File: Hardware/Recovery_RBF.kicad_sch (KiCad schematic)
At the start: 8 parts, among them J6 RCV_SYS, J7 RBF_SYS, Q8 AO3400A

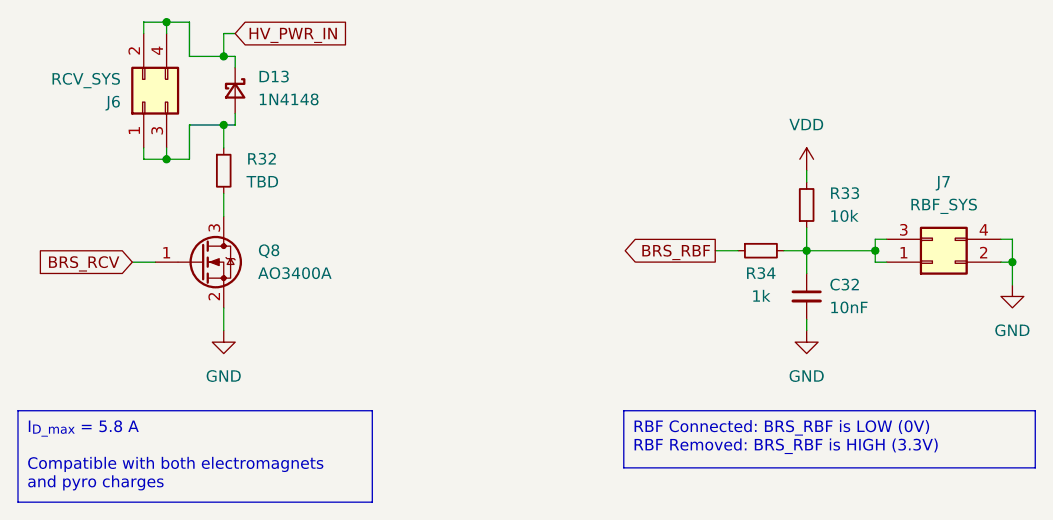
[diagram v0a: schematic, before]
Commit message: Developing HW - routing
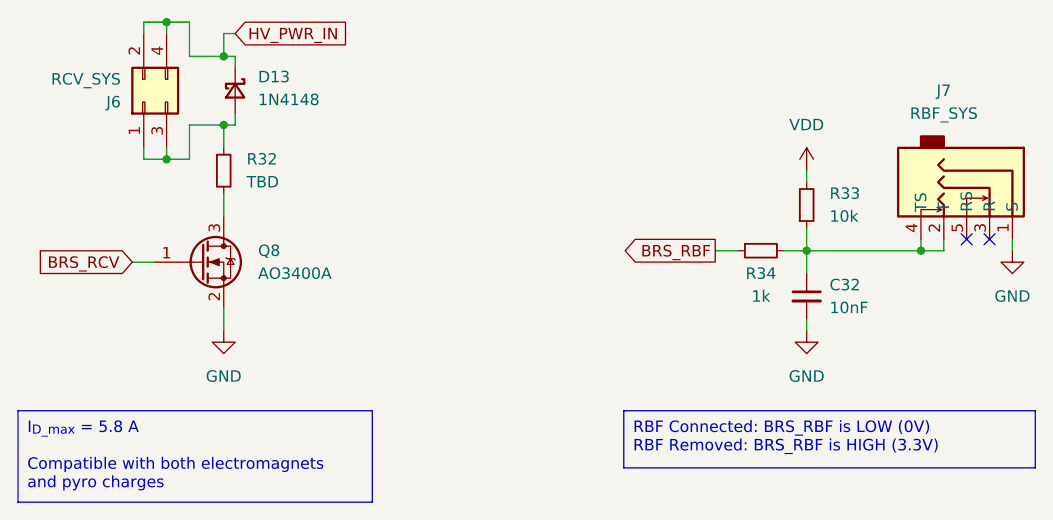
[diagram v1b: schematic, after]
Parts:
- J7: footprint Connector_Molex:Molex_Micro-Fit_3.0_43045-0412_2x02_P3.00mm_Vertical -> BRS_Footprints:AudioJack_Vertical; symbol Connector_Generic:Conn_02x02_Odd_Even -> BRS_Library:AudioJack_5pins
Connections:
- net GND: now also J7.1 (S); no longer J7.2 (Pin_2), J7.4 (Pin_4)
- net at C32.1, R33.1, R34.2: now also J7.2 (T), J7.4 (TS); no longer J7.1 (Pin_1), J7.3 (Pin_3)
- no-connect marks 0 -> 2
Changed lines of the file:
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@@
-	)
-	(junction
-		(at 191.77 101.6)
-		(diameter 0)
-		(color 0 0 0 0)
 	)
 	(junction
@@
 	)
 	(junction
-		(at 207.01 102.87)
-		(diameter 0)
-		(color 0 0 0 0)
-	)
-	(junction
 		(at 119.38 80.01)
 		(diameter 0)
 		(color 0 0 0 0)
 	)
+	(junction
+		(at 196.85 101.6)
+		(diameter 0)
+		(color 0 0 0 0)
+	)
+	(no_connect
+		(at 204.47 100.33)
+	)
+	(no_connect
+		(at 201.93 100.33)
+	)
 	(wire
 		(pts
@@
 	(wire
 		(pts
-			(xy 207.01 102.87) (xy 205.74 102.87)
-		)
-		(stroke
-			(width 0)
-			(type default)
-		)
-	)
-	(wire
-		(pts
-			(xy 207.01 100.33) (xy 205.74 100.33)
-		)
-		(stroke
-			(width 0)
-			(type default)
-		)
-	)
-	(wire
-		(pts
 			(xy 109.22 102.87) (xy 111.76 102.87)
 		)
@@
 	(wire
 		(pts
+			(xy 196.85 101.6) (xy 184.15 101.6)
+		)
+		(stroke
+			(width 0)
+			(type default)
+		)
+	)
+	(wire
+		(pts
 			(xy 120.65 81.28) (xy 120.65 80.01)
 		)
@@
 	(wire
 		(pts
-			(xy 184.15 101.6) (xy 191.77 101.6)
-		)
-		(stroke
-			(width 0)
-			(type default)
-		)
-	)
-	(wire
-		(pts
 			(xy 120.65 77.47) (xy 119.38 77.47)
 		)
@@
 	(wire
 		(pts
-			(xy 207.01 100.33) (xy 207.01 102.87)
+			(xy 199.39 101.6) (xy 196.85 101.6)
 		)
 		(stroke
@@
 	(wire
 		(pts
-			(xy 191.77 102.87) (xy 191.77 101.6)
-		)
-		(stroke
-			(width 0)
-			(type default)
-		)
-	)
-	(wire
-		(pts
-			(xy 193.04 102.87) (xy 191.77 102.87)
+			(xy 199.39 100.33) (xy 199.39 101.6)
 		)
 		(stroke
@@
 	(wire
 		(pts
-			(xy 191.77 100.33) (xy 193.04 100.33)
-		)
-		(stroke
-			(width 0)
-			(type default)
-		)
-	)
-	(wire
-		(pts
 			(xy 113.03 76.2) (xy 113.03 77.47)
 		)
@@
 	(wire
 		(pts
-			(xy 191.77 100.33) (xy 191.77 101.6)
-		)
-		(stroke
-			(width 0)
-			(type default)
-		)
-	)
-	(wire
-		(pts
 			(xy 119.38 107.95) (xy 119.38 110.49)
 		)
@@
 	(wire
 		(pts
+			(xy 196.85 100.33) (xy 196.85 101.6)
+		)
+		(stroke
+			(width 0)
+			(type default)
+		)
+	)
+	(wire
+		(pts
 			(xy 115.57 76.2) (xy 113.03 76.2)
 		)
@@
 	(wire
 		(pts
+			(xy 207.01 101.6) (xy 207.01 100.33)
+		)
+		(stroke
+			(width 0)
+			(type default)
+		)
+	)
+	(wire
+		(pts
 			(xy 110.49 91.44) (xy 113.03 91.44)
 		)
@@
 		(pts
 			(xy 115.57 87.63) (xy 115.57 91.44)
-		)
-		(stroke
-			(width 0)
-			(type default)
-		)
-	)
-	(wire
-		(pts
-			(xy 207.01 102.87) (xy 207.01 105.41)
 		)
 		(stroke
@@
 	)
 	(symbol
-		(lib_id "Connector_Generic:Conn_02x02_Odd_Even")
-		(at 198.12 102.87 0)
-		(mirror x)
+		(lib_id "BRS_Library:AudioJack_5pins")
+		(at 201.93 93.98 270)
 		(unit 1)
 		(exclude_from_sim no)
@@
 		(dnp no)
 		(property "Reference" "J7"
-			(at 199.39 93.98 0)
+			(at 199.39 83.82 90)
 			(effects
 				(font
@@
 		)
 		(property "Value" "RBF_SYS"
-			(at 199.39 96.52 0)
-			(effects
-				(font
-					(size 1.27 1.27)
-				)
-			)
-		)
-		(property "Footprint" "Connector_Molex:Molex_Micro-Fit_3.0_43045-0412_2x02_P3.00mm_Vertical"
-			(at 198.12 102.87 0)
+			(at 199.39 86.36 90)
+			(effects
+				(font
+					(size 1.27 1.27)
+				)
+			)
+		)
+		(property "Footprint" "BRS_Footprints:AudioJack_Vertical"
+			(at 201.93 93.98 0)
 			(effects
 				(font
@@
 		)
 		(property "Datasheet" "~"
-			(at 198.12 102.87 0)
-			(effects
-				(font
-					(size 1.27 1.27)
-				)
-				(hide yes)
-			)
-		)
-		(property "Description" "Generic connector, double row, 02x02, odd/even pin numbering scheme (row 1 odd numbers, row 2 even numbers), script generated (kicad-library-utils/schlib/autogen/connector/)"
-			(at 198.12 102.87 0)
-			(effects
-				(font
-					(size 1.27 1.27)
-				)
-				(hide yes)
-			)
+			(at 201.93 93.98 0)
+			(effects
+				(font
+					(size 1.27 1.27)
+				)
+				(hide yes)
+			)
+		)
+		(property "Description" "Audio Jack, 3 Poles (Stereo / TRS), Switched TR Poles (Normalling)"
+			(at 201.93 93.98 0)
+			(effects
+				(font
+					(size 1.27 1.27)
+				)
+				(hide yes)
+			)
+		)
+		(pin "5"
+		)
+		(pin "3"
+		)
+		(pin "1"
 		)
 		(pin "2"
 		)
-		(pin "1"
-		)
 		(pin "4"
-		)
-		(pin "3"
 		)
 		(instances
@@
 	(symbol
 		(lib_id "power:GND")
-		(at 207.01 105.41 0)
+		(at 207.01 101.6 0)
 		(unit 1)
 		(exclude_from_sim no)
@@
 		(dnp no)
 		(property "Reference" "#PWR096"
-			(at 207.01 111.76 0)
+			(at 207.01 107.95 0)
 			(effects
 				(font
@@
 		)
 		(property "Value" "GND"
-			(at 207.01 110.49 0)
+			(at 207.01 106.68 0)
 			(effects
 				(font
@@
 		)
 		(property "Footprint" ""
-			(at 207.01 105.41 0)
+			(at 207.01 101.6 0)
 			(effects
 				(font
@@
 		)
 		(property "Datasheet" ""
-			(at 207.01 105.41 0)
+			(at 207.01 101.6 0)
 			(effects
 				(font
@@
 		)
 		(property "Description" ""
-			(at 207.01 105.41 0)
-			(effects
-				(font
+			(at 207.01 101.6 0)
+			(effects
+				(font

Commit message: Working on power source
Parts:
- C32: footprint Capacitor_SMD:C_0603_1608Metric -> Capacitor_SMD:C_0402_1005Metric
- R32, R33, R34: footprint Resistor_SMD:R_0603_1608Metric -> Resistor_SMD:R_0402_1005Metric
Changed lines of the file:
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@@
 			)
 		)
-		(property "Footprint" "Resistor_SMD:R_0603_1608Metric"
+		(property "Footprint" "Resistor_SMD:R_0402_1005Metric"
 			(at 179.07 101.6 0)
 			(effects
@@
 			)
 		)
-		(property "Footprint" "Resistor_SMD:R_0603_1608Metric"
+		(property "Footprint" "Resistor_SMD:R_0402_1005Metric"
 			(at 184.15 96.52 0)
 			(effects
@@
 			)
 		)
-		(property "Footprint" "Resistor_SMD:R_0603_1608Metric"
+		(property "Footprint" "Resistor_SMD:R_0402_1005Metric"
 			(at 119.38 92.71 0)
 			(effects
@@
 			)
 		)
-		(property "Footprint" "Capacitor_SMD:C_0603_1608Metric"
+		(property "Footprint" "Capacitor_SMD:C_0402_1005Metric"
 			(at 184.15 106.68 0)
 			(effects
